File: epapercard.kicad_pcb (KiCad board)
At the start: 2 copper layers, 43 parts, among them P1 CONN_01X06, P2 A120699CT, Q1 2N7002KW, Q2 BSS84W, Q3 AP2305, Q4 BSS84W, Q5 2N7002KW, Q6 2N7002KW, Q7 2N7002KW, SW1 SW_PUSH, U1 MSP430G2553IPW20R

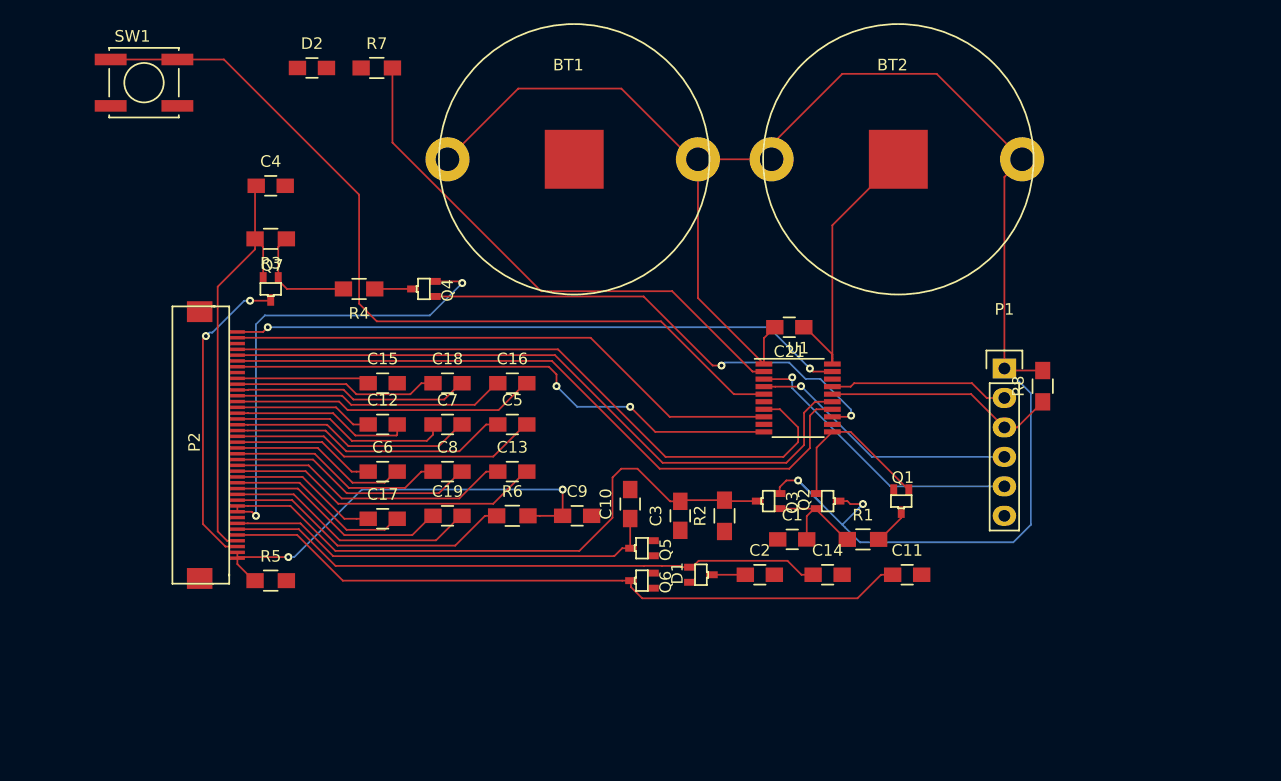
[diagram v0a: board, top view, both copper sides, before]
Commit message: I remembered how mirrors work
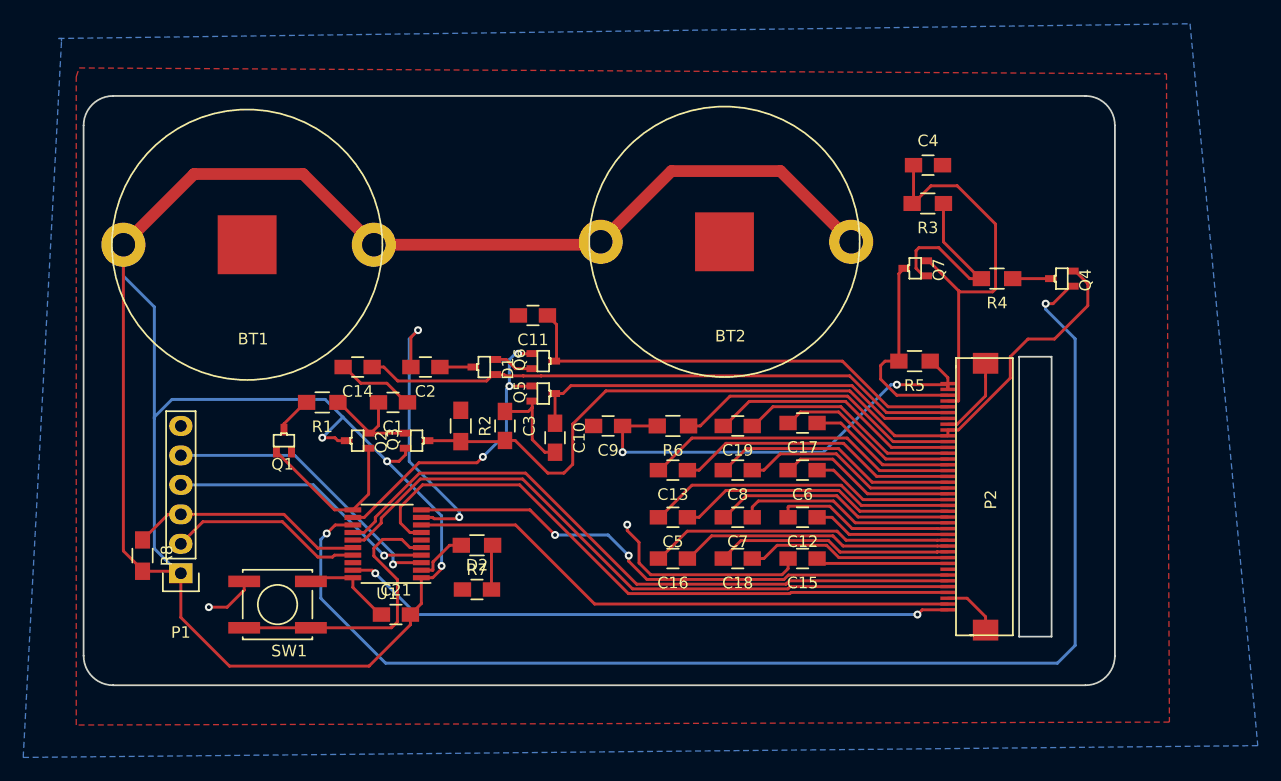
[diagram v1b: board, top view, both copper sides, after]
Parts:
- moved R8 79.0 mm to (28.6, 69.5), turned to 270 degrees
- moved P1 73.2 mm to (31.9, 71.0), turned to 180 degrees
- moved P2 71.4 mm to (103.0, 64.6), turned to 90 degrees
- moved R5 58.6 mm to (95.1, 52.7), turned to 180 degrees
- moved R3 56.7 mm to (96.3, 39.1)
- moved C4 56.7 mm to (96.3, 35.8)
- moved Q7 55.6 mm to (95.2, 44.7), turned to 270 degrees
- moved R4 55.0 mm to (102.2, 45.6)
- moved Q4 55.0 mm to (107.8, 45.6)
- moved Q1 53.5 mm to (40.8, 59.6), turned to 180 degrees
- moved R1 48.1 mm to (44.1, 56.3), turned to 180 degrees
- moved D2 47.2 mm to (57.4, 72.4)
- moved SW1 46.4 mm to (40.2, 73.7), turned to 180 degrees
- moved C14 44.3 mm to (47.1, 53.2), turned to 180 degrees
- moved R7 42.0 mm to (57.4, 68.6), turned to 180 degrees
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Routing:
- net BORDER_CONTROL: track 42.3 -> 109.9 mm
- net +3V3: track 154.4 -> 210.3 mm, vias 2 -> 3
- net /button: track 73.8 -> 25.3 mm
- net /led: track 46.6 -> 4.74 mm
- net GND: track 24.3 -> 61.2 mm, vias 0 -> 2
- net DISCHARGE: track 0.00 -> 26.9 mm, vias 0 -> 3
- net PWM: track 0.00 -> 25.0 mm, vias 0 -> 2
- net /VDH: track 59.9 -> 39.9 mm
- net +3.3VP: track 93.1 -> 74.4 mm, vias 2 -> 0
- net /BORDER: track 27.0 -> 17.5 mm, vias 2 -> 0
- net Net-(Q7-Pad1): track 9.79 -> 17.4 mm
- net Net-(D2-Pad2): track 0.00 -> 3.85 mm
- net SPI_CLK: track 57.6 -> 55.4 mm
- net /test: track 15.5 -> 17.0 mm
- net SPI_MOSI: track 58.9 -> 57.7 mm
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- added copper zone on B.Cu, net GND
- added copper zone on F.Cu, net GND
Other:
- board outline added: 88.9 x 50.8 mm
- net class Default: trace_width 0.1524 -> 0.254
- board text added: "CUT OUT"
- board text added: "Paul Schow"
- board text added: "paulschow.com"
- board text added: "paulschow@gmail.com"
